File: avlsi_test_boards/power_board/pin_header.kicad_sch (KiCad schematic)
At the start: 4 parts, among them J5 Conn_02x20_Odd_Even, J6 Conn_02x20_Odd_Even, J7 Conn_02x20_Odd_Even, J8 Conn_02x20_Odd_Even

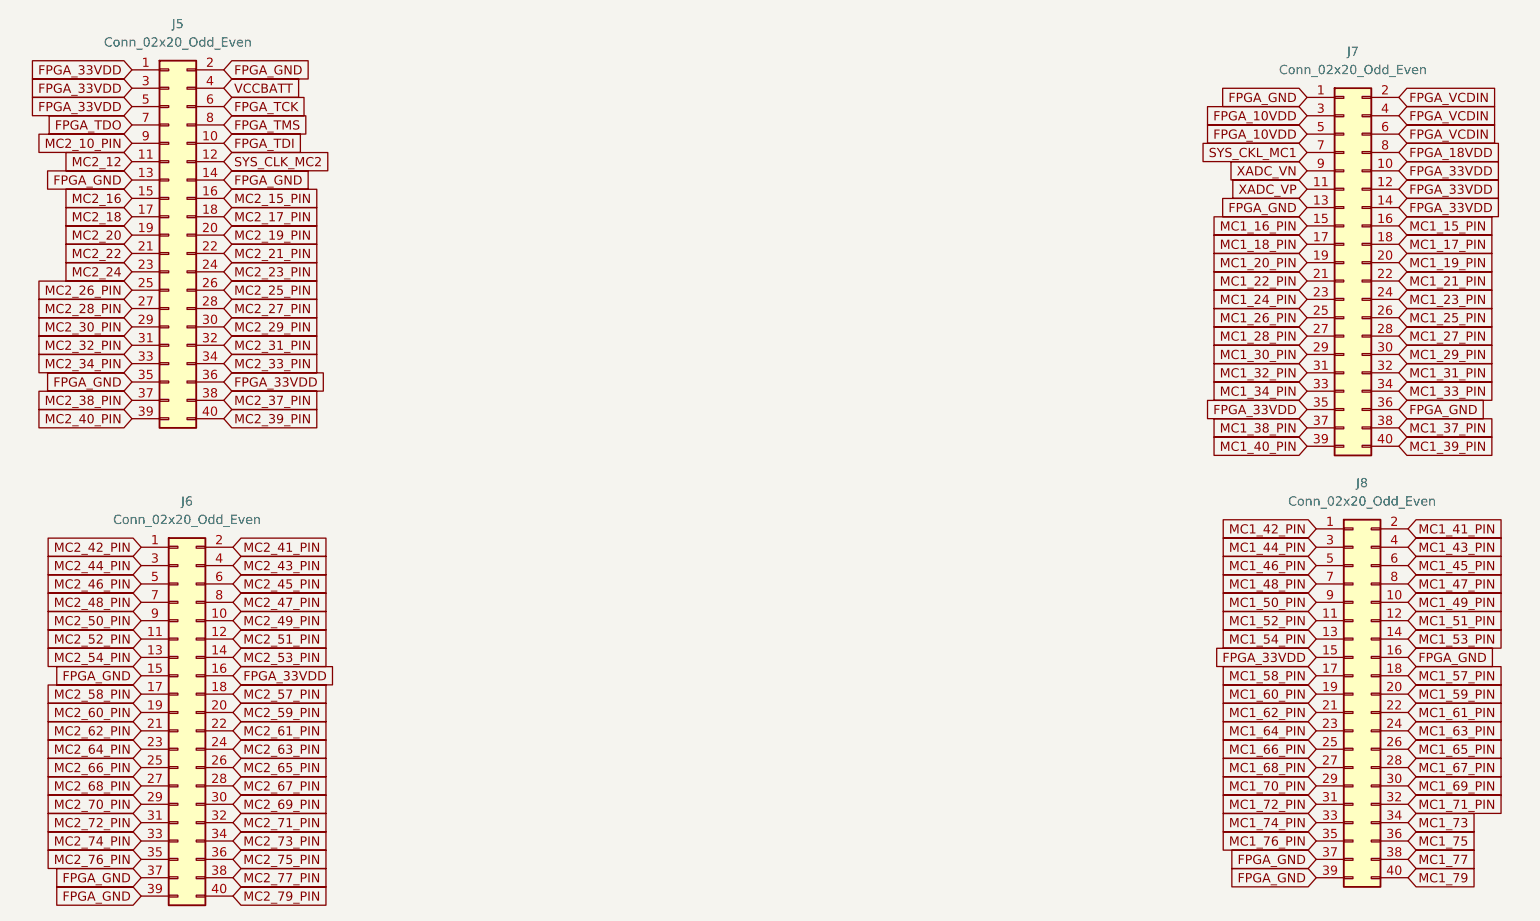
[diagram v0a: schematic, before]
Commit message: progress
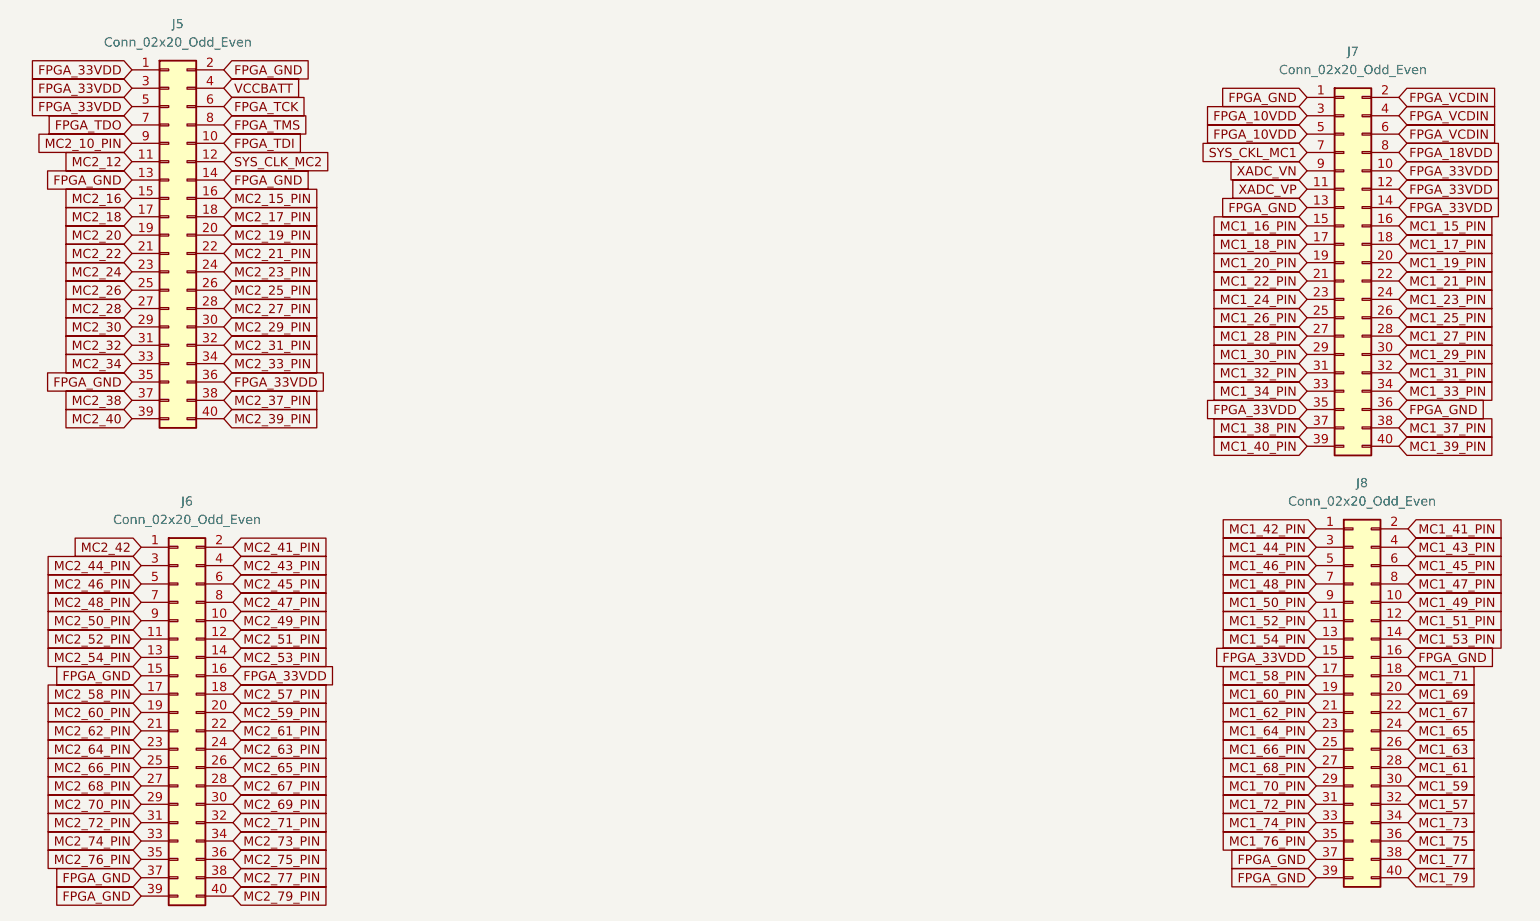
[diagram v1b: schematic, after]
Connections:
- net MC1_57_PIN renamed MC1_71
- net MC1_59_PIN renamed MC1_69
- net MC1_61_PIN renamed MC1_67
- net MC1_63_PIN renamed MC1_65
- net MC1_65_PIN renamed MC1_63
- net MC1_67_PIN renamed MC1_61
- net MC1_69_PIN renamed MC1_59
- net MC1_71_PIN renamed MC1_57
- net MC2_26_PIN renamed MC2_26
- net MC2_28_PIN renamed MC2_28
- net MC2_30_PIN renamed MC2_30
- net MC2_32_PIN renamed MC2_32
- net MC2_34_PIN renamed MC2_34
- net MC2_38_PIN renamed MC2_38
- net MC2_40_PIN renamed MC2_40
- net MC2_42_PIN renamed MC2_42
